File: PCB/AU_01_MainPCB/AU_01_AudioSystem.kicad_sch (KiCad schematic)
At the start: 4 parts, among them U4 ADAU1701, U5 PAM8320RDR, U6 PAM8302AASCR, U7 PAM8302AASCR

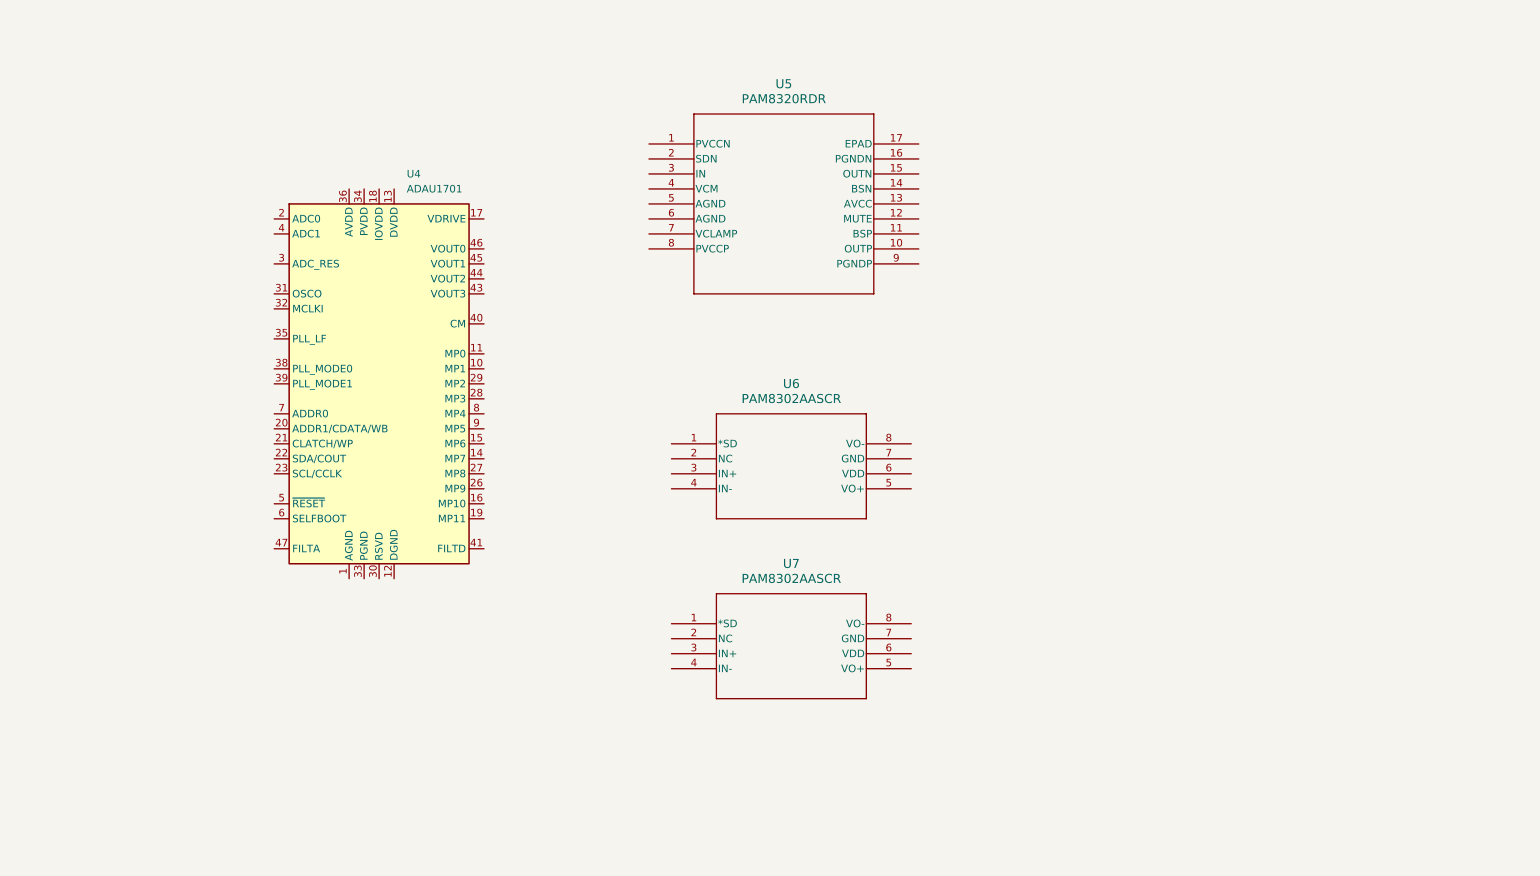
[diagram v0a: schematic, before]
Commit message: Audio, Battery Schematic, added Journal
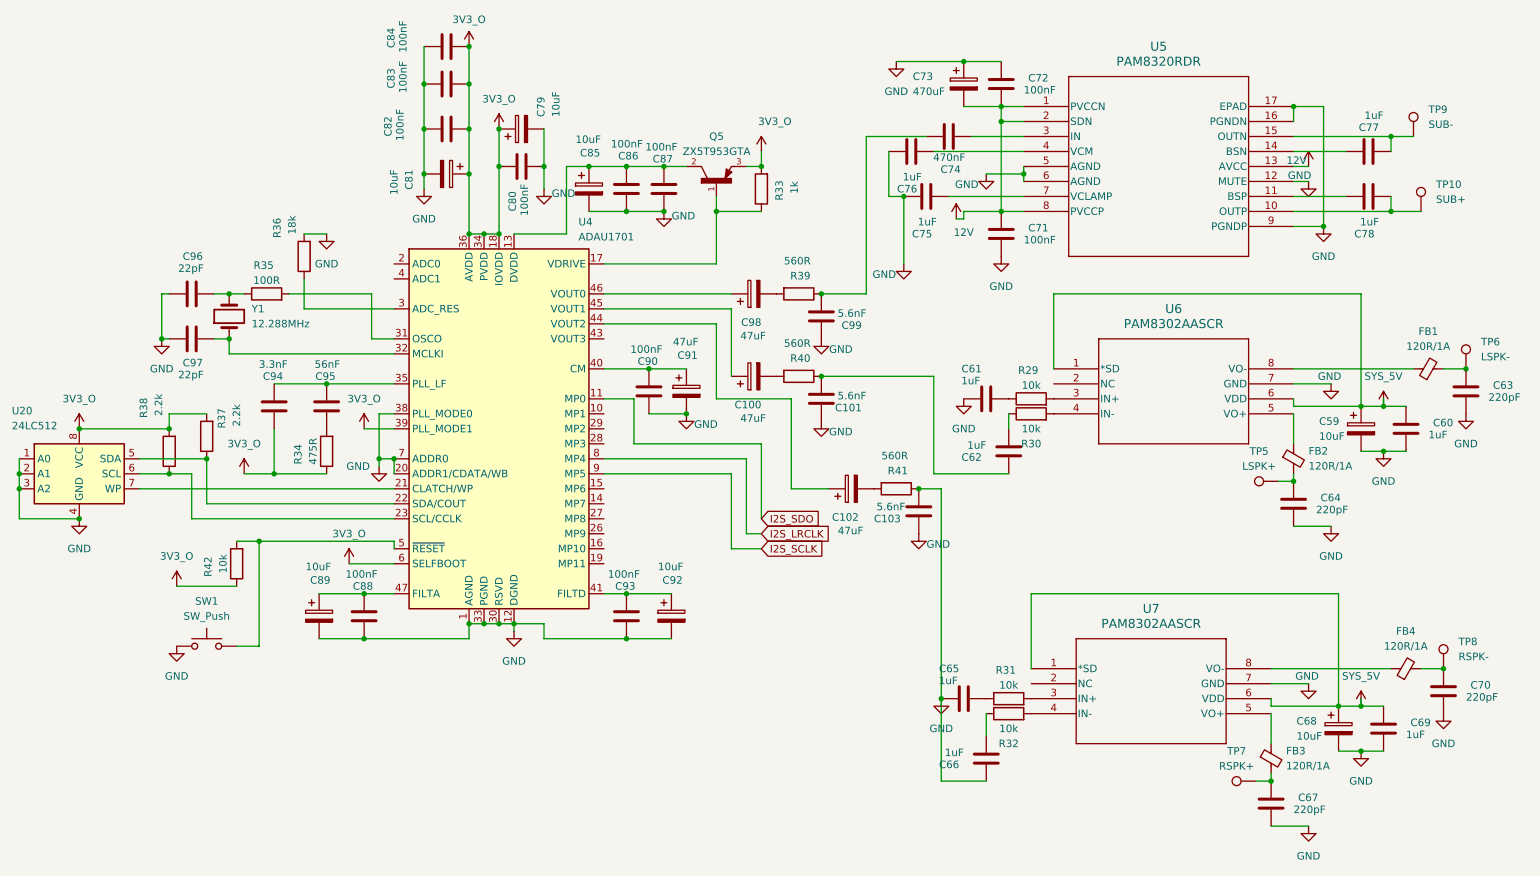
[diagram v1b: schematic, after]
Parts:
- added C100, C102, C91, C98: 47uF, symbol Device:C_Polarized
- added C101, C103, C99: 5.6nF, symbol Device:C
- added C59, C68, C79, C81, C85, C89, C92: 10uF, symbol Device:C_Polarized
- added C60, C61, C62, C65, C66, C69, C75, C76, C77, C78: 1uF, symbol Device:C
- added C63, C64, C67, C70: 220pF, symbol Device:C
- added C71, C72, C80, C82, C83, C84, C86, C87, C88, C90, C93: 100nF, symbol Device:C
- added C73: 470uF, symbol Device:C_Polarized
- added C74: 470nF, symbol Device:C
- added C94: 3.3nF, symbol Device:C
- added C95: 56nF, symbol Device:C
- added C96, C97: 22pF, symbol Device:C
- added FB1, FB2, FB3, FB4: 120R/1A, symbol Device:FerriteBead_Small
- added Q5: ZX5T953GTA, ZX5T953GTA:SOT230P700X180-4N, symbol ZX5T953:ZX5T953GTA
- added R29, R30, R31, R32, R42: 10k, symbol Device:R
- added R33: 1k, symbol Device:R
- added R34: 475R, symbol Device:R
- added R35: 100R, symbol Device:R
- added R36: 18k, symbol Device:R
- added R37, R38: 2.2k, symbol Device:R
- added R39, R40, R41: 560R, symbol Device:R
- added SW1: SW_Push, symbol Switch:SW_Push
- added TP10: SUB+, symbol Connector:TestPoint
- added TP5: LSPK+, symbol Connector:TestPoint
- added TP6: LSPK-, symbol Connector:TestPoint
- added TP7: RSPK+, symbol Connector:TestPoint
- added TP8: RSPK-, symbol Connector:TestPoint
- added TP9: SUB-, symbol Connector:TestPoint
- added U20: 24LC512, symbol Memory_EEPROM:24LC512
- added Y1: 12.288MHz, symbol Device:Crystal
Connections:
- net GND: now reaches U4.1 (AGND), U4.37 (AGND), U4.42 (AGND)
- net GND: now also U4.12 (DGND), U4.20 (ADDR1/CDATA/WB), U4.25 (DGND), U4.30 (RSVD), U4.33 (PGND), U4.38 (PLL_MODE0), U4.7 (ADDR0), U5.12 (MUTE), U5.16 (PGNDN), U5.17 (EPAD), U5.5 (AGND), U5.6 (AGND), U5.9 (PGNDP), U6.7 (GND), U7.7 (GND), C101.1, C103.1, C103.2, C59.2, C60.2, C61.1, C63.2, C64.2, C65.1, C66.1, C67.2, C68.2, C69.2, C70.2, C71.2, C72.1, C73.1, C75.1, C76.1, C79.2, C80.2, C81.2, C82.1, C83.1, C84.1, C85.2, C86.1, C87.1, C88.1, C89.2, C90.1, C91.2, C92.2, C93.1, C96.2, C97.2, C99.1, R36.2, R41.1, SW1.1, U20.1 (A0), U20.2 (A1), U20.3 (A2), U20.4 (GND)
- net I2S_SDO: now reaches U4.11 (MP0)
- net at U4.13 (DVDD), U4.24 (DVDD): now also C85.1, C86.2, C87.2, Q5.2, Q5.4
- net at U4.17 (VDRIVE): now also Q5.1, R33.1
- net 3V3_O: now reaches U4.18 (IOVDD)
- net 3V3_O: now also U4.34 (PVDD), U4.36 (AVDD), U4.39 (PLL_MODE1), U4.48 (AVDD), U4.6 (SELFBOOT), C79.1, C80.1, C81.1, C82.2, C83.2, C84.2, C94.1, Q5.3, R33.2, R34.1, R37.2, R38.2, R42.1, U20.8 (VCC)
- net at U4.21 (CLATCH/WP): now also U20.7 (WP)
- net at U4.22 (SDA/COUT): now also R37.1, U20.5 (SDA)
- net at U4.23 (SCL/CCLK): now also R38.1, U20.6 (SCL)
- net at U4.3 (ADC_RES): now also R36.1
- net at U4.31 (OSCO): now also R35.2
- net at U4.32 (MCLKI): now also C97.1, Y1.1
- net at U4.35 (PLL_LF): now also C94.2, C95.2
- net at U4.40 (CM): now also C90.2, C91.1
- net at U4.41 (FILTD): now also C92.1, C93.2
- net at U4.44 (VOUT2): now also C102.1
- net at U4.45 (VOUT1): now also C100.1
- net at U4.46 (VOUT0): now also C98.1
- net at U4.47 (FILTA): now also C88.2, C89.1
- net at U4.5 (~{RESET}): now also R42.2, SW1.2
- net I2S_LRCLK: now reaches U4.8 (MP4)
- net I2S_SCLK: now reaches U4.9 (MP5)
- net SYS_5V: now reaches U6.1 (*SD)
- net SYS_5V: now also U6.6 (VDD), U7.1 (*SD), U7.6 (VDD), C59.1, C60.1, C68.1, C69.1
- net at U6.3 (IN+): now also R29.2
- net at U6.4 (IN-): now also R30.2
- net at U6.5 (VO+): now also FB2.1
- net at U6.8 (VO-): now also FB1.1
- net 12V: now reaches U5.1 (PVCCN)
- net 12V: now also U5.13 (AVCC), U5.2 (SDN), U5.8 (PVCCP), C71.1, C72.2, C73.2
- net at U5.10 (OUTP): now also C78.2, TP10.1
- net at U5.11 (BSP): now also C78.1
- net at U5.14 (BSN): now also C77.1
- net at U5.15 (OUTN): now also C77.2, TP9.1
- net at U5.3 (IN): now also C74.2
- net at U5.4 (VCM): now also C76.2
- net at U5.7 (VCLAMP): now also C75.2
- net at U7.3 (IN+): now also R31.2
- net at U7.4 (IN-): now also R32.2
- net at U7.5 (VO+): now also FB3.1
- net at U7.8 (VO-): now also FB4.1
- new net: C67.1, FB3.2, TP7.1
- new net: C95.1, R34.2
- new net: C101.2, C62.1, R40.1
- new net: C62.2, R30.1
- new net: C100.2, R40.2
- new net: C102.2, R41.2
- new net: C96.1, R35.1, Y1.2
- new net: C64.1, FB2.2, TP5.1
- new net: C70.1, FB4.2, TP8.1
- new net: C61.2, R29.1
- new net: C63.1, FB1.2, TP6.1
- new net: C66.2, R32.1
- new net: C98.2, R39.2
- new net: C74.1, C99.2, R39.1
- new net: C65.2, R31.1
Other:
- moved on the sheet: U4, U5, U6
